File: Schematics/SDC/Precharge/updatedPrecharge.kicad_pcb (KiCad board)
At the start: 2 copper layers, 34.3 x 26.2 mm, 14 parts, among them J1 Conn_01x06, Q1 VN3205N3-G, Q2 VP3203N3-G, Q4 VP3203N3-G, U1 LM358DR2G

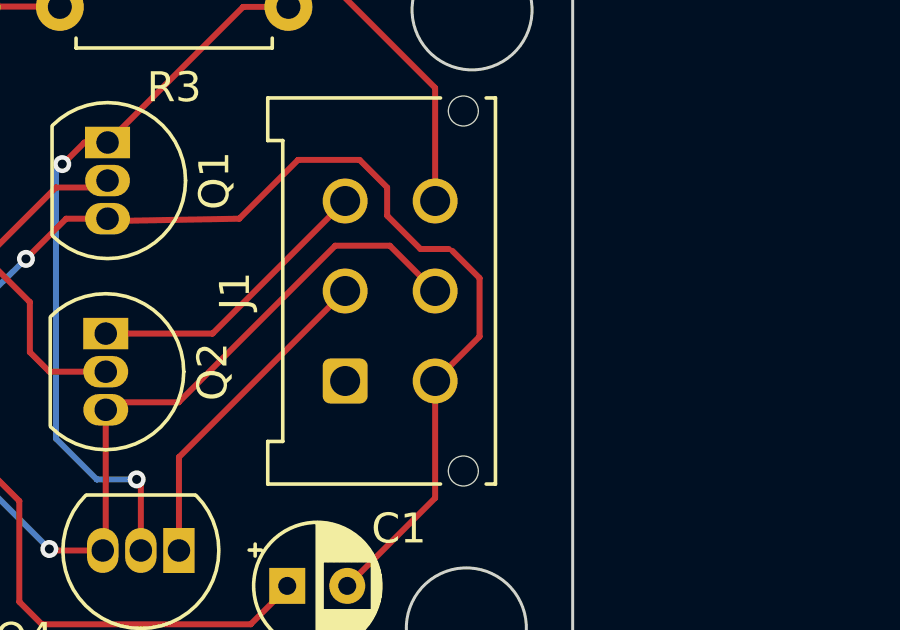
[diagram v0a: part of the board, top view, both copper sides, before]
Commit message: fixed up boards
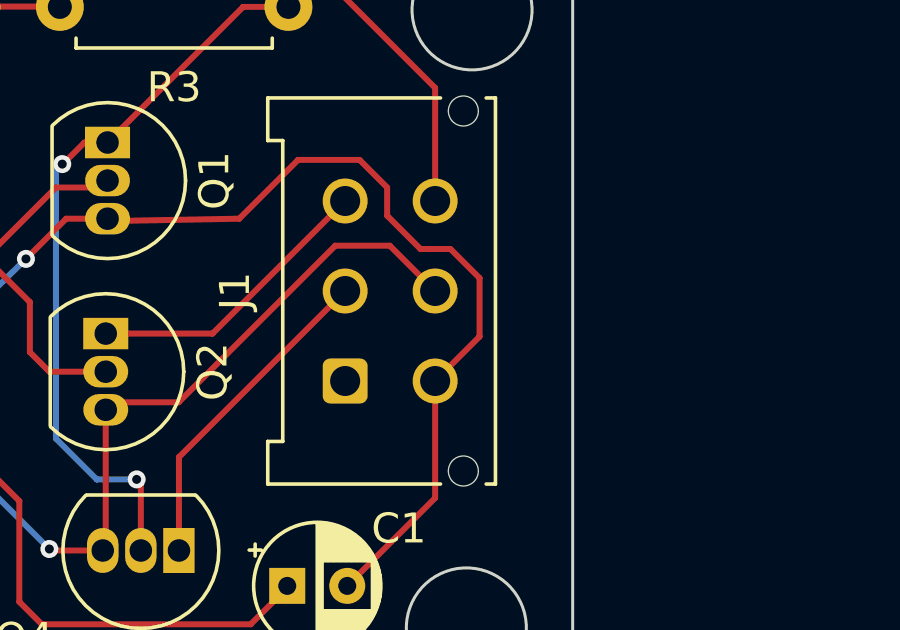
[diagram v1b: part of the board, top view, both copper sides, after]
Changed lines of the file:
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@@
   (segment (start 116.81 122.66) (end 116.16 122.01) (width 0.2) (layer "F.Cu") (net 6))
   (segment (start 114.685 118.865) (end 117.03 116.52) (width 0.2) (layer "F.Cu") (net 6))
-  (segment (start 131.15 121.49) (end 131.15 119.54) (width 0.2) (layer "F.Cu") (net 7))
-  (segment (start 118.76 117.64) (end 123.14 117.56) (width 0.2) (layer "F.Cu") (net 7))
   (segment (start 123.14 117.56) (end 125.1 115.6) (width 0.2) (layer "F.Cu") (net 7))
   (segment (start 107.815 121.405) (end 109.655 121.405) (width 0.2) (layer "F.Cu") (net 7))
@@
   (segment (start 107.815 123.905) (end 107.98 124.07) (width 0.2) (layer "F.Cu") (net 7))
   (segment (start 109.655 121.405) (end 109.71 121.46) (width 0.2) (layer "F.Cu") (net 7))
-  (segment (start 127.15 115.6) (end 128.07 116.52) (width 0.2) (layer "F.Cu") (net 7))
-  (segment (start 131.15 119.54) (end 130.24 118.63) (width 0.2) (layer "F.Cu") (net 7))
-  (segment (start 129.67 122.97) (end 131.15 121.49) (width 0.2) (layer "F.Cu") (net 7))
+  (segment (start 118.76 117.64) (end 123.14 117.56) (width 0.2) (layer "F.Cu") (net 7))
+  (segment (start 129.18 118.57) (end 130.18 118.57) (width 0.2) (layer "F.Cu") (net 7))
   (segment (start 118.75 117.56) (end 117.37 117.56) (width 0.2) (layer "F.Cu") (net 7))
-  (segment (start 128.07 117.46) (end 129.18 118.57) (width 0.2) (layer "F.Cu") (net 7))
-  (segment (start 129.18 118.57) (end 130.13 118.57) (width 0.2) (layer "F.Cu") (net 7))
   (segment (start 129.67 126.87) (end 126.74 129.8) (width 0.2) (layer "F.Cu") (net 7))
   (segment (start 129.67 122.97) (end 129.67 126.87) (width 0.2) (layer "F.Cu") (net 7))
+  (segment (start 118.75 117.56) (end 118.76 117.64) (width 0.2) (layer "F.Cu") (net 7))
+  (segment (start 125.1 115.6) (end 127.15 115.6) (width 0.2) (layer "F.Cu") (net 7))
+  (segment (start 131.15 121.49) (end 129.67 122.97) (width 0.2) (layer "F.Cu") (net 7))
   (segment (start 101.82 129.13) (end 106.42 129.13) (width 0.2) (layer "F.Cu") (net 7))
-  (segment (start 125.1 115.6) (end 127.15 115.6) (width 0.2) (layer "F.Cu") (net 7))
+  (segment (start 130.18 118.57) (end 131.15 119.54) (width 0.2) (layer "F.Cu") (net 7))
   (segment (start 106.42 129.13) (end 106.5 129.21) (width 0.2) (layer "F.Cu") (net 7))
   (segment (start 100.89 124.79) (end 100.89 128.2) (width 0.2) (layer "F.Cu") (net 7))
-  (segment (start 128.07 116.52) (end 128.07 117.46) (width 0.2) (layer "F.Cu") (net 7))
+  (segment (start 131.15 119.54) (end 131.15 121.49) (width 0.2) (layer "F.Cu") (net 7))
   (segment (start 106.62 122.6) (end 107.815 121.405) (width 0.2) (layer "F.Cu") (net 7))
   (segment (start 103.08 122.6) (end 100.89 124.79) (width 0.2) (layer "F.Cu") (net 7))
-  (segment (start 118.75 117.56) (end 118.76 117.64) (width 0.2) (layer "F.Cu") (net 7))
+  (segment (start 128.07 117.46) (end 129.18 118.57) (width 0.2) (layer "F.Cu") (net 7))
   (segment (start 109.73 121.48) (end 109.67 121.42) (width 0.2) (layer "F.Cu") (net 7))
+  (segment (start 127.15 115.6) (end 128.07 116.52) (width 0.2) (layer "F.Cu") (net 7))
+  (segment (start 128.07 116.52) (end 128.07 117.46) (width 0.2) (layer "F.Cu") (net 7))
   (segment (start 107.815 121.405) (end 107.815 123.905) (width 0.2) (layer "F.Cu") (net 7))
   (via (at 116.03 118.9) (size 0.6) (drill 0.3) (layers "F.Cu" "B.Cu") (net 7))
